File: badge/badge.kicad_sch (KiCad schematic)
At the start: 8 parts, among them SW1 SW_Push, U1 TPS7250QP

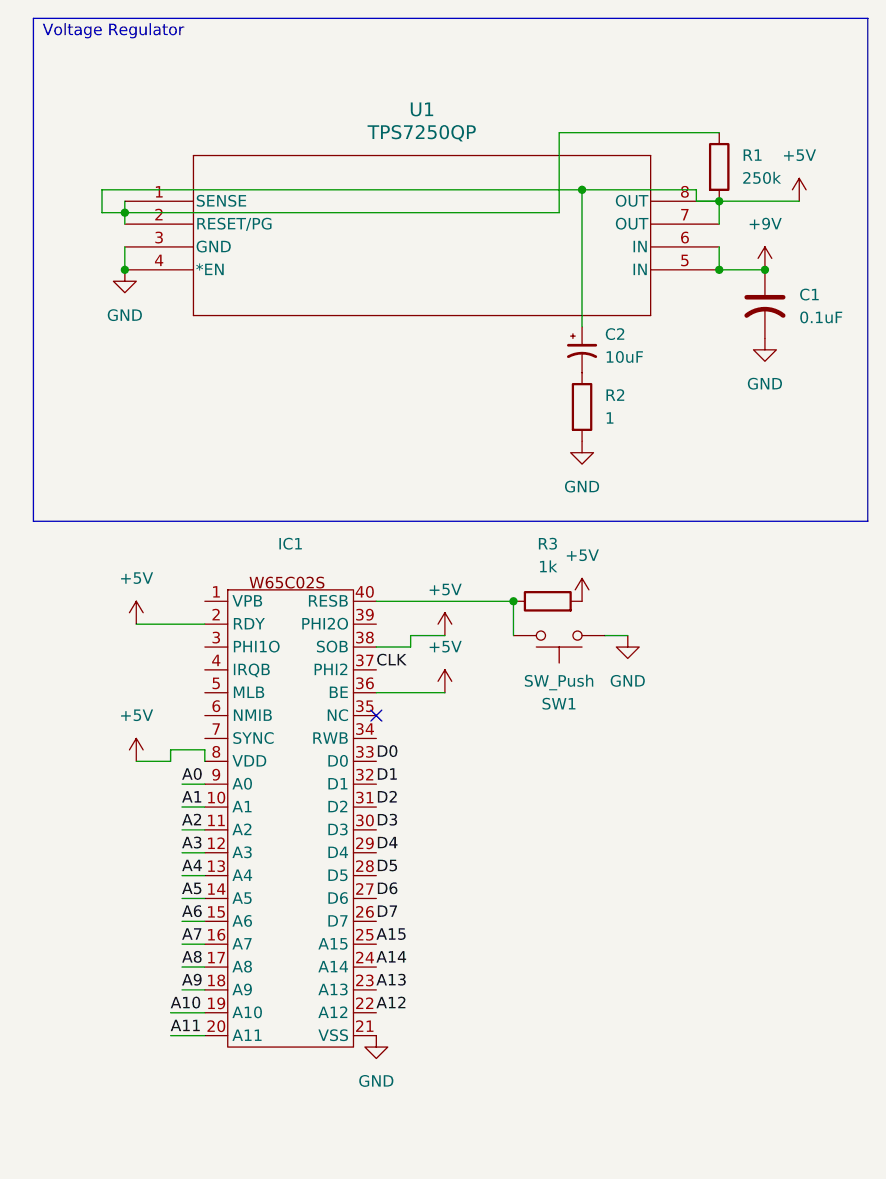
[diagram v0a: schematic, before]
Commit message: Make the voltage regulator look nice
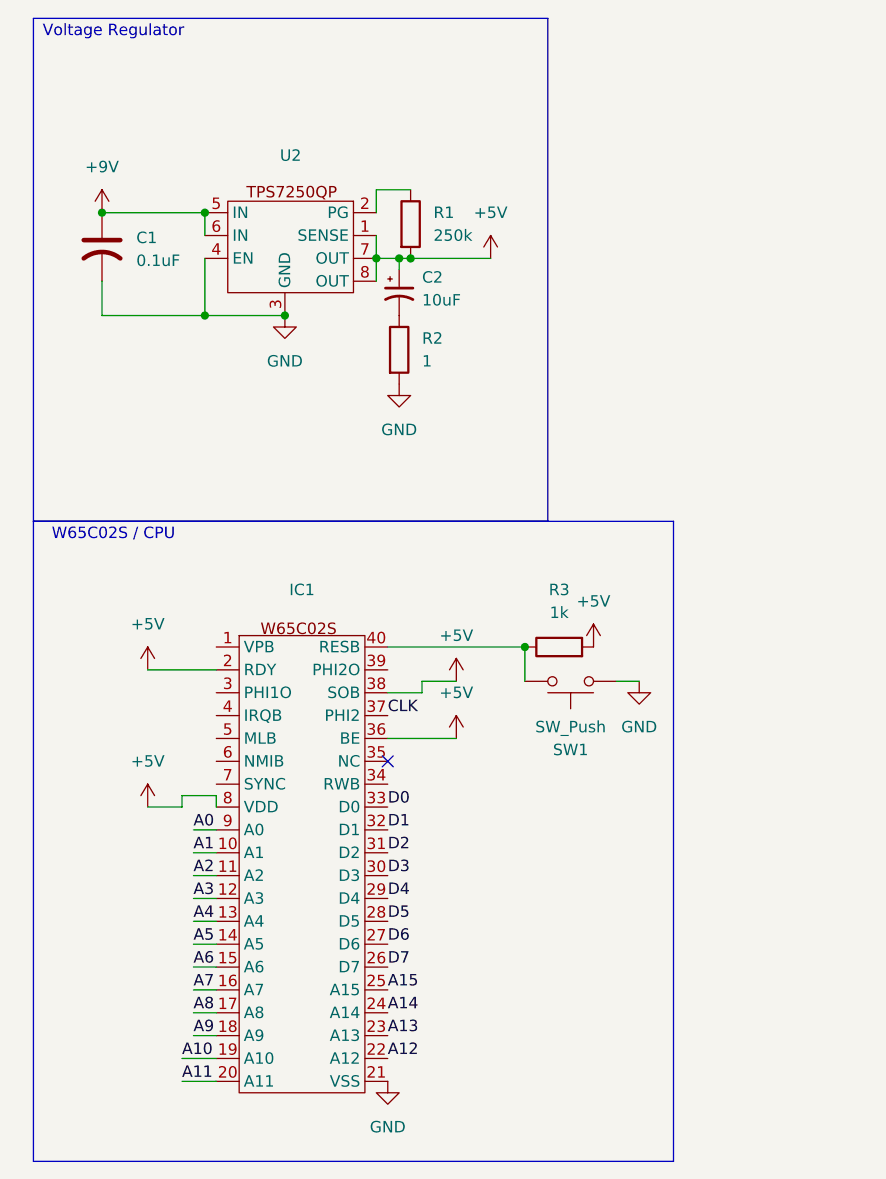
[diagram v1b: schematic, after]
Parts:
- removed U1: TPS7250QP, P8_TEX, symbol TPS7250QP:TPS7250QP
- added U2: ~, symbol 6502ConferenceBadge:TPS7250QP
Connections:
- net +5V: now also U2.1 (SENSE), U2.7 (OUT), U2.8 (OUT); no longer R1.1
- net +9V: now also U2.5 (IN), U2.6 (IN)
- net GND: now also U2.3 (GND), U2.4 (EN)
- new net: R1.1, U2.2 (PG)
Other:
- note added: "W65C02S / CPU"
- moved on the sheet: IC1, R3, SW1
